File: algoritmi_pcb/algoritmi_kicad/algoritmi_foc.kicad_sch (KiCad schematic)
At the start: 25 parts, among them IC2 AP2114HA-3.3TRG1, J2 53261-0371, J3 SMM-110-02-H-D-K-TR, U1 TMC6300-LA-T

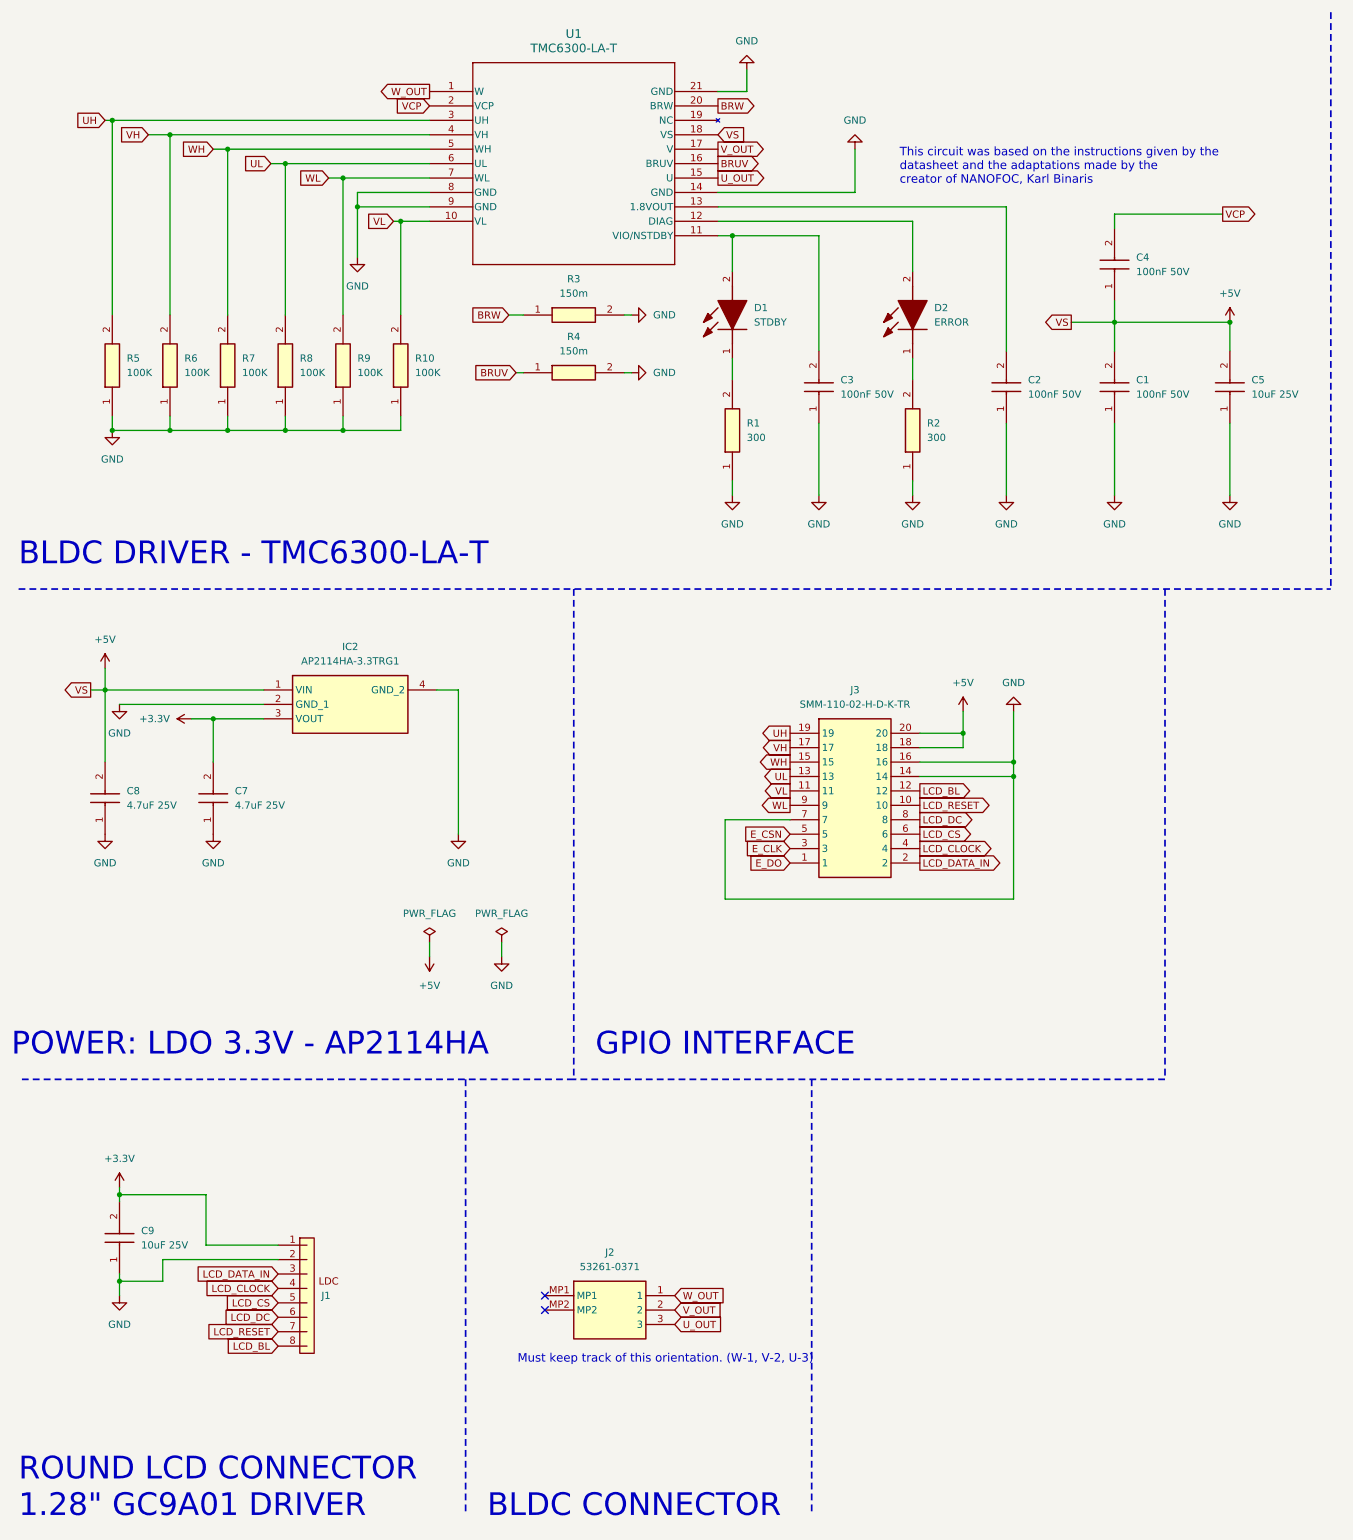
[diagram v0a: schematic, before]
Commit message: some changes to schematics
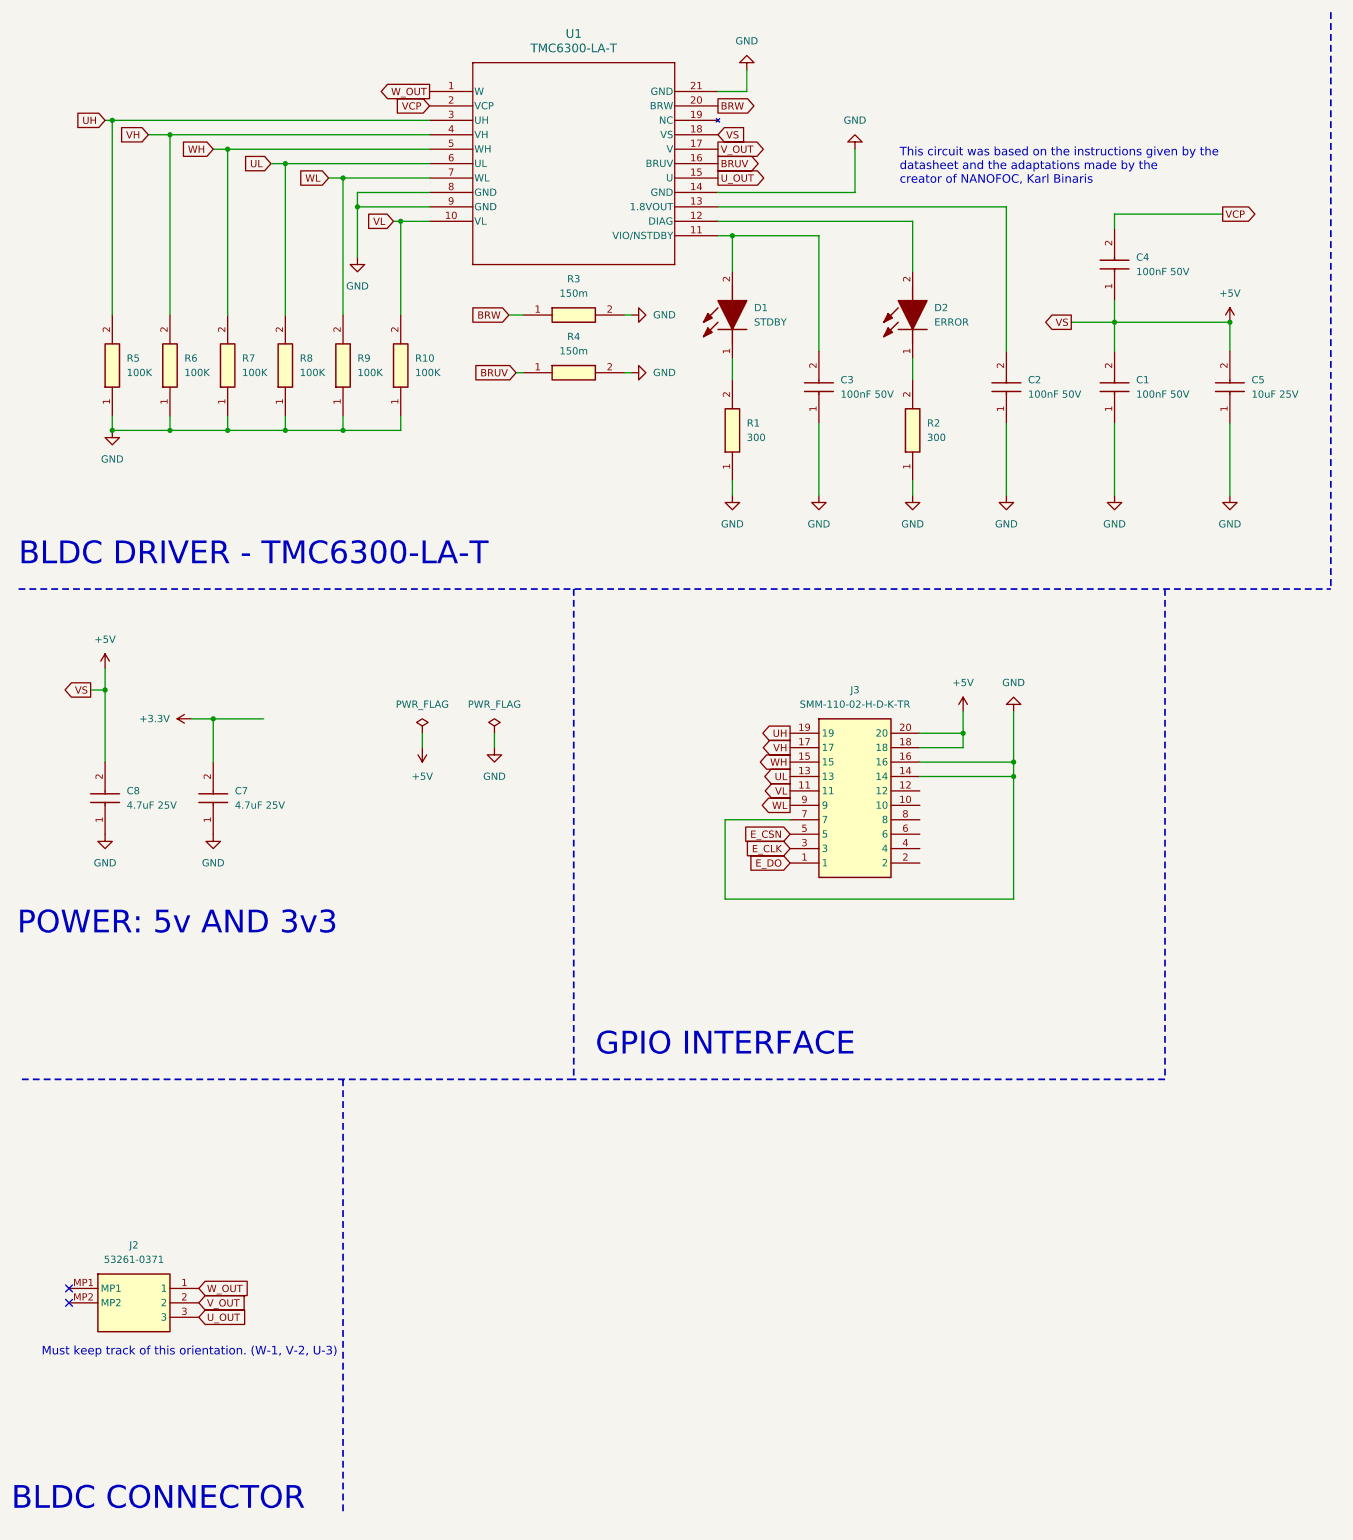
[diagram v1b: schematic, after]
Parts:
- removed C9: 10uF 25V, Capacitor_SMD:C_0805_2012Metric, symbol SamacSys_Parts:CL21A106KAYNNNE
- removed IC2: AP2114HA-3.3TRG1, Package_TO_SOT_SMD:SOT-223-3_TabPin2, symbol SamacSys_Parts:AP2114HA-3.3TRG1
- removed J1: ~, solder_pads:solder_pads_2mm_8, symbol solder_pad:solder_pad_2mm_8
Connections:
- net LCD_BL: no longer names the net of J3.12
- net LCD_CLOCK: no longer names the net of J3.4
- net LCD_CS: no longer names the net of J3.6
- net LCD_DATA_IN: no longer names the net of J3.2
- net LCD_DC: no longer names the net of J3.8
- net LCD_RESET: no longer names the net of J3.10
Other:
- note added: "POWER: 5v AND 3v3"
- note removed: "POWER: LDO 3.3V - AP2114HA"
- note removed: "ROUND LCD CONNECTOR 1.28" GC9A01 DRIVER"
- moved on the sheet: J2
